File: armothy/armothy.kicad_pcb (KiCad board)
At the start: 2 copper layers, 90.2 x 59.7 mm, 21 parts, among them J1 I2C, J2 UART, J3 motZ, J4 pump, J5 valve, J6 Encoder, J7 Limit switch, J8 12V_PWR, J9 Conn_01x03_Female, U1 L293D, U2 Teensy3.2, U3 TSR_1-2450, U4 LM7810_TO220

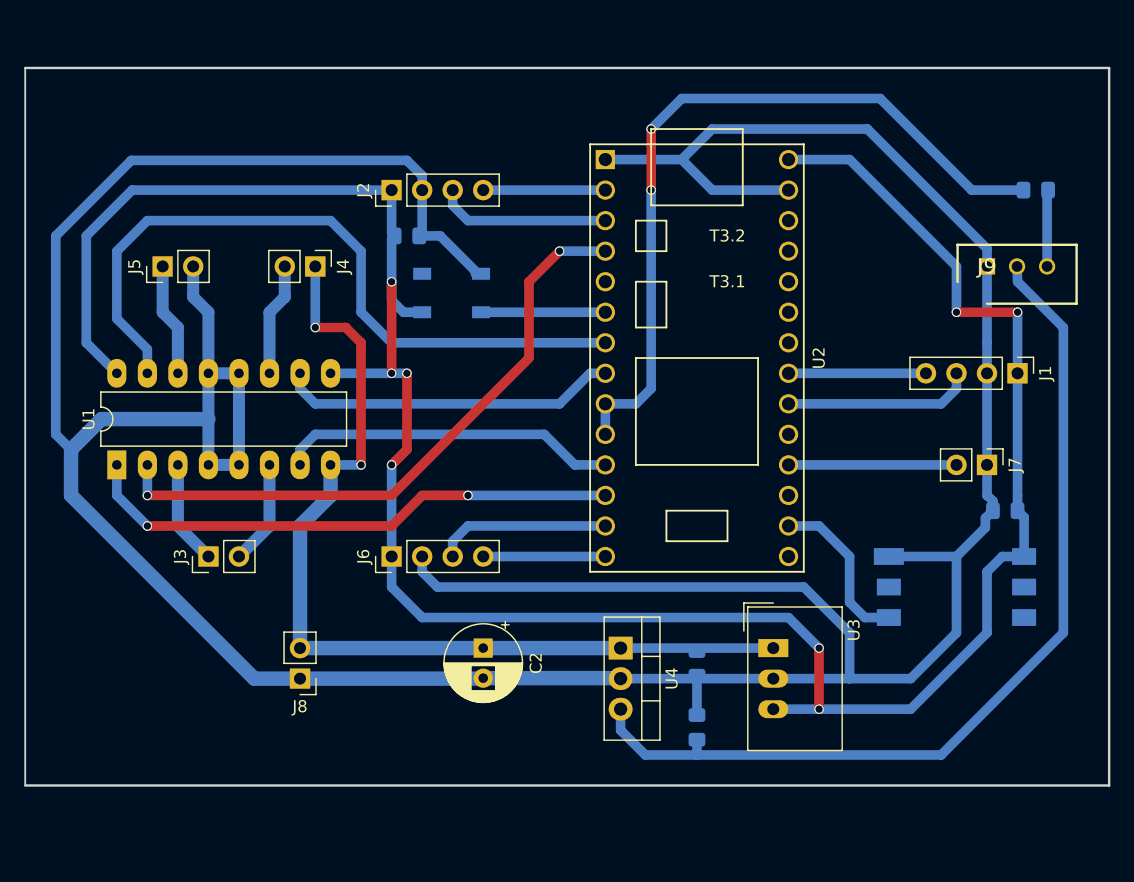
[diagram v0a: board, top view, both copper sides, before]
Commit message: Armothy controller V2.0
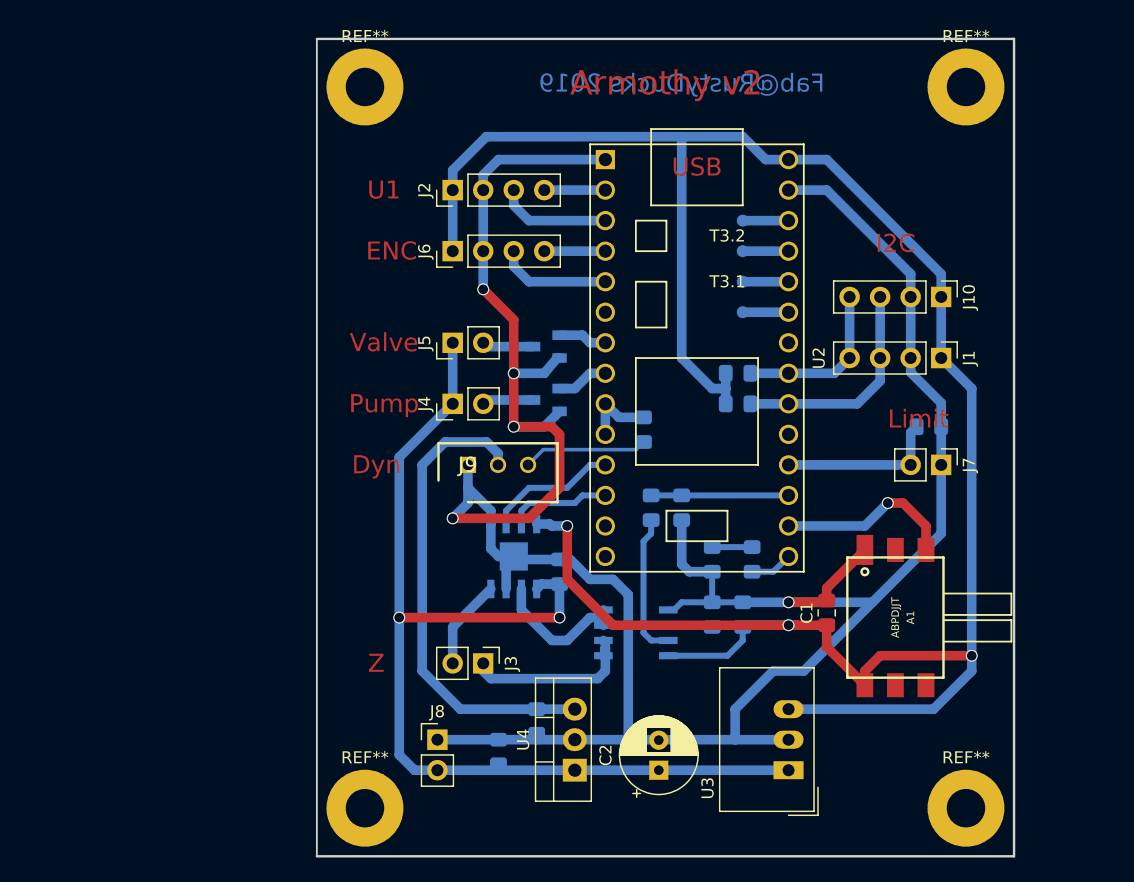
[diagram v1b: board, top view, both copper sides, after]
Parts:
- removed U1: L293D, Package_DIP:DIP-16_W7.62mm_LongPads
- added C6: 100n, Capacitor_SMD:C_0805_2012Metric_Pad1.15x1.40mm_HandSolder, B.Cu at (138.4, 103.9)
- added C7: 100n, Capacitor_SMD:C_0805_2012Metric_Pad1.15x1.40mm_HandSolder, B.Cu at (135.9, 103.9)
- added C8: 100n, Capacitor_SMD:C_0805_2012Metric_Pad1.15x1.40mm_HandSolder, B.Cu at (123.2, 100.3)
- added J10: I2C, Connector_PinHeader_2.54mm:PinHeader_1x04_P2.54mm_Vertical, F.Cu at (154.9, 77.5)
- added Q1: IRL6283M, mosfets:SOT-23, B.Cu at (122.1, 81.6)
- added Q2: IRL6283M, mosfets:SOT-23, B.Cu at (122.1, 86.0)
- added R3: 2.2K, Resistor_SMD:R_0805_2012Metric_Pad1.15x1.40mm_HandSolder, B.Cu at (138.0, 83.8)
- added R4: 2.2K, Resistor_SMD:R_0805_2012Metric_Pad1.15x1.40mm_HandSolder, B.Cu at (138.0, 86.4)
- added R5: 5K, Resistor_SMD:R_0805_2012Metric_Pad1.15x1.40mm_HandSolder, B.Cu at (130.8, 95.0)
- added R6: 10K, Resistor_SMD:R_0805_2012Metric_Pad1.15x1.40mm_HandSolder, B.Cu at (133.3, 95.0)
- added R7: 100, Resistor_SMD:R_0805_2012Metric_Pad1.15x1.40mm_HandSolder, B.Cu at (139.2, 99.3)
- added REF**: MountingHole_3.2mm_M3_Pad, MountingHole:MountingHole_3.2mm_M3_Pad, F.Cu at (157.0, 60.0)
- added REF**: MountingHole_3.2mm_M3_Pad, MountingHole:MountingHole_3.2mm_M3_Pad, F.Cu at (107.0, 120.0)
- added REF**: MountingHole_3.2mm_M3_Pad, MountingHole:MountingHole_3.2mm_M3_Pad, F.Cu at (107.0, 60.0)
- added REF**: MountingHole_3.2mm_M3_Pad, MountingHole:MountingHole_3.2mm_M3_Pad, F.Cu at (157.0, 120.0)
- added TP1: TestPoint, TestPoint:TestPoint_Pad_D1.0mm, B.Cu at (138.4, 71.1)
- added TP2: TestPoint, TestPoint:TestPoint_Pad_D1.0mm, B.Cu at (138.4, 73.7)
- added TP3: TestPoint, TestPoint:TestPoint_Pad_D1.0mm, B.Cu at (138.4, 78.7)
- added TP4: TestPoint, TestPoint:TestPoint_Pad_D1.0mm, B.Cu at (138.4, 76.2)
- added U5: ACS712xLCTR-05B, Package_SO:SOIC-8_3.9x4.9mm_P1.27mm, B.Cu at (129.5, 105.4)
- added U6: A4953_LJ, Package_SO:SOIC-8-1EP_3.9x4.9mm_P1.27mm_EP2.35x2.35mm, B.Cu at (119.4, 99.1)
- A1, C1: moved to F.Cu
- D1: value WS2812B -> LED; footprint leds:LED_WS2812B_5.0x5.0mm -> LED_SMD:LED_0805_2012Metric_Pad1.15x1.40mm_HandSolder
- moved C5 46.2 mm to (153.9, 88.3)
- moved J9 46.2 mm to (115.6, 91.4)
- moved R1 38.2 mm to (130.2, 88.5), turned to 90 degrees
- moved D1 31.0 mm to (135.9, 99.3), turned to 90 degrees
- moved J6 25.9 mm to (114.3, 73.7)
- moved J5 25.0 mm to (114.3, 81.3)
- moved J3 24.5 mm to (116.8, 108.0), turned to 270 degrees
- moved C3 18.1 mm to (118.1, 115.3), turned to 90 degrees
- moved C2 17.8 mm to (131.4, 116.8), turned to 90 degrees
- moved C1 17.1 mm to (145.4, 103.8), turned to 90 degrees
- moved J4 16.2 mm to (114.3, 86.4), turned to 90 degrees
- moved C4 13.3 mm to (121.3, 112.8), turned to 270 degrees
- moved J8 12.5 mm to (113.0, 114.3), turned to 0 degrees
- moved U4 10.9 mm to (124.5, 116.8), turned to 90 degrees
- moved U3 10.2 mm to (142.2, 116.8), turned to 90 degrees
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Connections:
- A1 pad 2: Net-(A1-Pad2) -> (no net)
- A1 pad 4: Net-(A1-Pad4) -> (no net)
- A1 pad 5: Net-(A1-Pad5) -> (no net)
- C2 pad 1: /POWER -> +12V
- C3 pad 1: /POWER -> +12V
- C5 pad 1: +5V -> /LIM_SWITCH
- D1 pad 1: +5V -> GND
- J4 pad 1: /POWER -> +12V
- J5 pad 1: Net-(J5-Pad1) -> +12V
- J5 pad 2: GND -> Net-(J5-Pad2)
- J8 pad 2: /POWER -> +12V
- U2 pad 12: /MOTORZ_PWM -> /MOTORZ_A
- U2 pad 13: /ENC_A -> (no net)
- U2 pad 14: /ENC_B -> (no net)
- U2 pad 20: Net-(U2-Pad20) -> /STATUS_LED
- U2 pad 22: Net-(U2-Pad22) -> /Z_CURRENT
- U2 pad 24: Net-(U2-Pad24) -> (no net)
- U2 pad 27: Net-(U2-Pad27) -> (no net)
- U2 pad 4: /MOTORZ_A -> /ENC_B
- U2 pad 5: Net-(U2-Pad5) -> /ENC_A
- U2 pad 6: /RGB_LED -> (no net)
- U3 pad 1: /POWER -> +12V
- U4 pad 1: /POWER -> +12V
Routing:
- net GND: track 323.5 -> 224.5 mm, vias 0 -> 5
- net +12V: track 0.00 -> 87.7 mm, vias 0 -> 2
- net /POWER: track 77.8 -> 0.00 mm, vias 2 -> 0
- net /RX_DYN: track 63.6 -> 6.18 mm, vias 2 -> 0
- net /VALVE_CTRL: track 60.1 -> 4.07 mm
- net /MOTORZ_PWM: track 45.3 -> 0.00 mm, vias 2 -> 0
- net /MOTORZ_A: track 52.8 -> 8.62 mm, vias 2 -> 0
- net +10V: track 77.0 -> 39.6 mm
- net /PUMP_CTRL: track 28.2 -> 4.34 mm
- net /MOTORZ_B: track 28.2 -> 10.9 mm
- net +5V: track 203.0 -> 189.0 mm, vias 8 -> 3
- net Net-(R5-Pad1): track 0.00 -> 12.0 mm
- net Net-(U5-Pad3): track 0.00 -> 11.7 mm
- net /Z_CURRENT: track 0.00 -> 11.4 mm
- net /RGB_LED: track 10.3 -> 0.00 mm
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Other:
- board size 90.2 x 59.7 mm -> 58 x 68 mm
- net class Default: via_dia 0.8 -> 1; via_drill 0.6 -> 0.8
- board text added: "Armothy v2"
- board text added: "Dyn"
- board text added: "ENC"
- board text added: "Fab@RustyDucks 2019"
- board text added: "I2C"
- board text added: "Limit"
- board text added: "Pump"
- board text added: "U1"
- board text added: "USB"
- board text added: "Valve"
- board text added: "Z"
